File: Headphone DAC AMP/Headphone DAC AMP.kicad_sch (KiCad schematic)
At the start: 2 parts, among them J3 SJ-3502-SMT

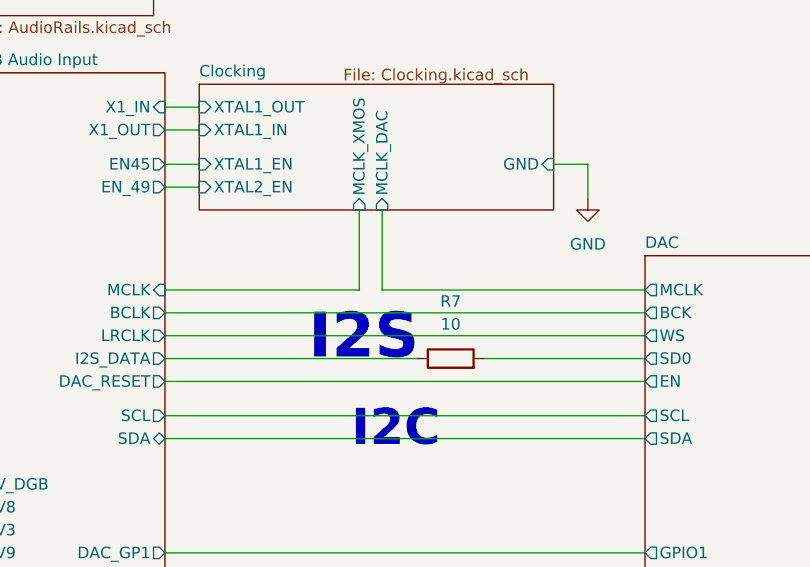
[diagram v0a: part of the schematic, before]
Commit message: Litterally didnt add anything because I spent an hour trying to understand how impedance matching works
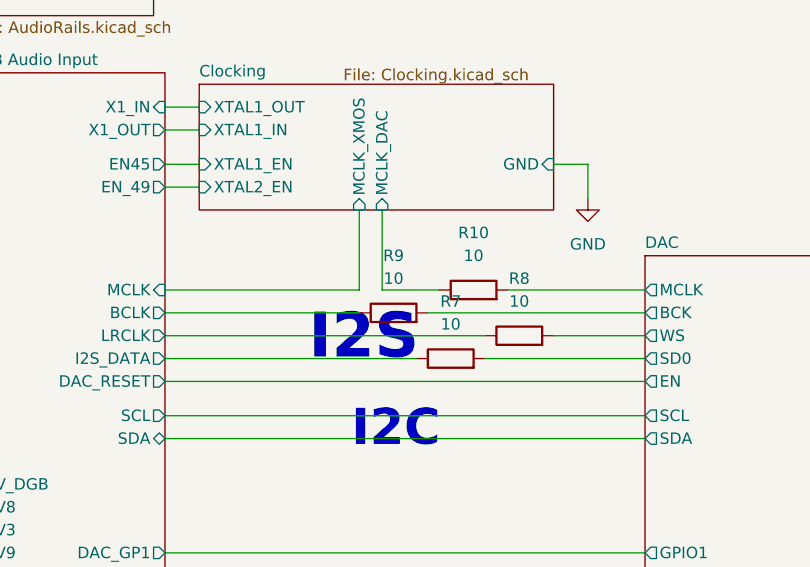
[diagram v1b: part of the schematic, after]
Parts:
- added R10, R8, R9: 10, Resistor_SMD:R_0805_2012Metric_Pad1.20x1.40mm_HandSolder, symbol Device:R
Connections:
- net Clocking/MCLK_DAC: now also R10.1
- net DAC/BCK: now also R9.2
- net DAC/WS: now also R8.2
- new net DAC/MCLK: R10.2
- new net USB Audio Input/BCLK: R9.1
- new net USB Audio Input/LRCLK: R8.1
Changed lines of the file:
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@@
 	(wire
 		(pts
-			(xy 90.17 76.2) (xy 143.51 76.2)
+			(xy 90.17 76.2) (xy 125.73 76.2)
 		)
 		(stroke
@@
 	(wire
 		(pts
-			(xy 90.17 73.66) (xy 143.51 73.66)
+			(xy 90.17 73.66) (xy 111.76 73.66)
 		)
 		(stroke
@@
 	(wire
 		(pts
-			(xy 114.3 71.12) (xy 143.51 71.12)
+			(xy 114.3 71.12) (xy 120.65 71.12)
 		)
 		(stroke
@@
 	(wire
 		(pts
+			(xy 133.35 76.2) (xy 143.51 76.2)
+		)
+		(stroke
+			(width 0)
+			(type default)
+		)
+	)
+	(wire
+		(pts
 			(xy 90.17 148.59) (xy 100.33 148.59)
 		)
@@
 	(wire
 		(pts
+			(xy 119.38 73.66) (xy 143.51 73.66)
+		)
+		(stroke
+			(width 0)
+			(type default)
+		)
+	)
+	(wire
+		(pts
 			(xy 90.17 85.09) (xy 143.51 85.09)
+		)
+		(stroke
+			(width 0)
+			(type default)
+		)
+	)
+	(wire
+		(pts
+			(xy 128.27 71.12) (xy 143.51 71.12)
 		)
 		(stroke
@@
 	)
 	(symbol
+		(lib_id "Device:R")
+		(at 129.54 76.2 90)
+		(unit 1)
+		(exclude_from_sim no)
+		(in_bom yes)
+		(on_board yes)
+		(dnp no)
+		(fields_autoplaced yes)
+		(property "Reference" "R8"
+			(at 129.54 69.85 90)
+			(effects
+				(font
+					(size 1.27 1.27)
+				)
+			)
+		)
+		(property "Value" "10"
+			(at 129.54 72.39 90)
+			(effects
+				(font
+					(size 1.27 1.27)
+				)
+			)
+		)
+		(property "Footprint" "Resistor_SMD:R_0805_2012Metric_Pad1.20x1.40mm_HandSolder"
+			(at 129.54 77.978 90)
+			(effects
+				(font
+					(size 1.27 1.27)
+				)
+				(hide yes)
+			)
+		)
+		(property "Datasheet" "~"
+			(at 129.54 76.2 0)
+			(effects
+				(font
+					(size 1.27 1.27)
+				)
+				(hide yes)
+			)
+		)
+		(property "Description" "Resistor"
+			(at 129.54 76.2 0)
+			(effects
+				(font
+					(size 1.27 1.27)
+				)
+				(hide yes)
+			)
+		)
+		(pin "1"
+		)
+		(pin "2"
+		)
+		(instances
+			(project "Headphone DAC AMP"
+				(path "/d034eddd-efbc-47be-a25c-37cbfbab4cd8"
+					(reference "R8")
+					(unit 1)
+				)
+			)
+		)
+	)
+	(symbol
 		(lib_id "power:GND")
 		(at 74.93 170.18 0)
@@
 	)
 	(symbol
+		(lib_id "Device:R")
+		(at 115.57 73.66 90)
+		(unit 1)
+		(exclude_from_sim no)
+		(in_bom yes)
+		(on_board yes)
+		(dnp no)
+		(fields_autoplaced yes)
+		(property "Reference" "R9"
+			(at 115.57 67.31 90)
+			(effects
+				(font
+					(size 1.27 1.27)
+				)
+			)
+		)
+		(property "Value" "10"
+			(at 115.57 69.85 90)
+			(effects
+				(font
+					(size 1.27 1.27)
+				)
+			)
+		)
+		(property "Footprint" "Resistor_SMD:R_0805_2012Metric_Pad1.20x1.40mm_HandSolder"
+			(at 115.57 75.438 90)
+			(effects
+				(font
+					(size 1.27 1.27)
+				)
+				(hide yes)
+			)
+		)
+		(property "Datasheet" "~"
+			(at 115.57 73.66 0)
+			(effects
+				(font
+					(size 1.27 1.27)
+				)
+				(hide yes)
+			)
+		)
+		(property "Description" "Resistor"
+			(at 115.57 73.66 0)
+			(effects
+				(font
+					(size 1.27 1.27)
+				)
+				(hide yes)
+			)
+		)
+		(pin "1"
+		)
+		(pin "2"
+		)
+		(instances
+			(project "Headphone DAC AMP"
+				(path "/d034eddd-efbc-47be-a25c-37cbfbab4cd8"
+					(reference "R9")
+					(unit 1)
+				)
+			)
+		)
+	)
+	(symbol
 		(lib_id "power:GND")
 		(at 203.2 93.98 0)
@@
 					(unit 1)
 				)
+			)
+		)
+	)
+	(symbol
+		(lib_id "Device:R")
+		(at 124.46 71.12 90)
+		(unit 1)
+		(exclude_from_sim no)
+		(in_bom yes)
+		(on_board yes)
+		(dnp no)
+		(fields_autoplaced yes)
+		(property "Reference" "R10"
+			(at 124.46 64.77 90)
+			(effects
+				(font
+					(size 1.27 1.27)
+				)
+			)
+		)
+		(property "Value" "10"
+			(at 124.46 67.31 90)
+			(effects
+				(font
+					(size 1.27 1.27)
+				)
+			)
+		)
+		(property "Footprint" "Resistor_SMD:R_0805_2012Metric_Pad1.20x1.40mm_HandSolder"
+			(at 124.46 72.898 90)
+			(effects
+				(font
+					(size 1.27 1.27)
+				)
+				(hide yes)
+			)
+		)
+		(property "Datasheet" "~"
+			(at 124.46 71.12 0)
+			(effects
+				(font
+					(size 1.27 1.27)
+				)
+				(hide yes)
+			)
+		)
+		(property "Description" "Resistor"
+			(at 124.46 71.12 0)
+			(effects
+				(font
+					(size 1.27 1.27)
+				)
+				(hide yes)
+			)
+		)
+		(pin "1"
+		)
+		(pin "2"
+		)
+		(instances
+			(project "Headphone DAC AMP"
+				(path "/d034eddd-efbc-47be-a25c-37cbfbab4cd8"
+					(reference "R10")
+					(unit 1)
+				)
